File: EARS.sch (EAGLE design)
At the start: 7 parts, among them IC1 STM32L152RDT

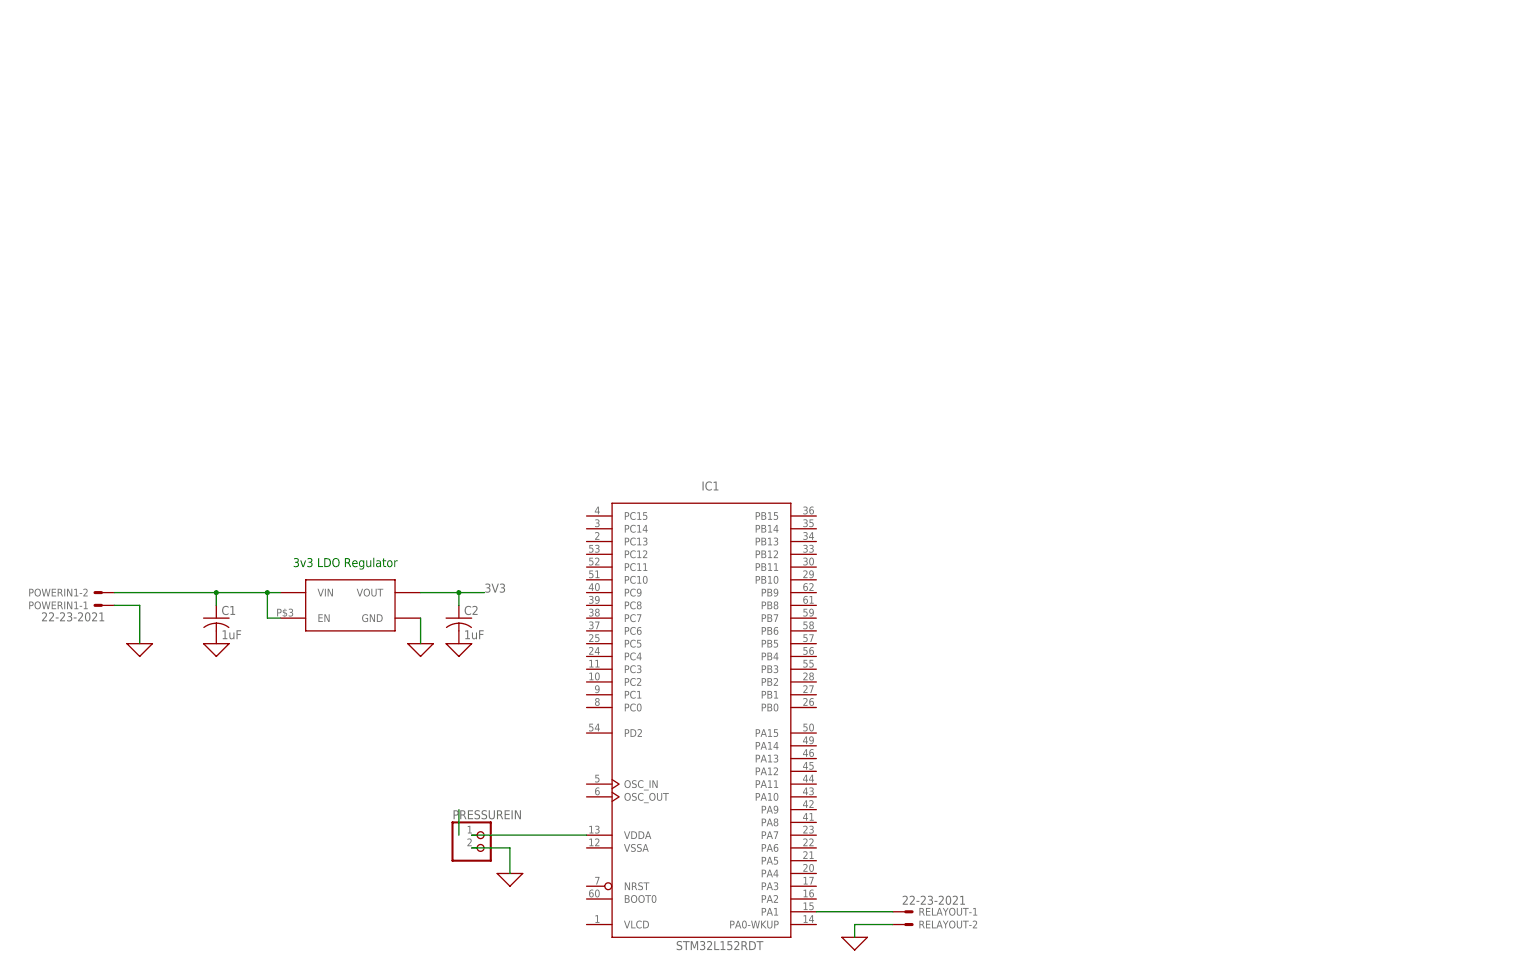
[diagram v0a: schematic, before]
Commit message: Initial Layout, fixed schematic.
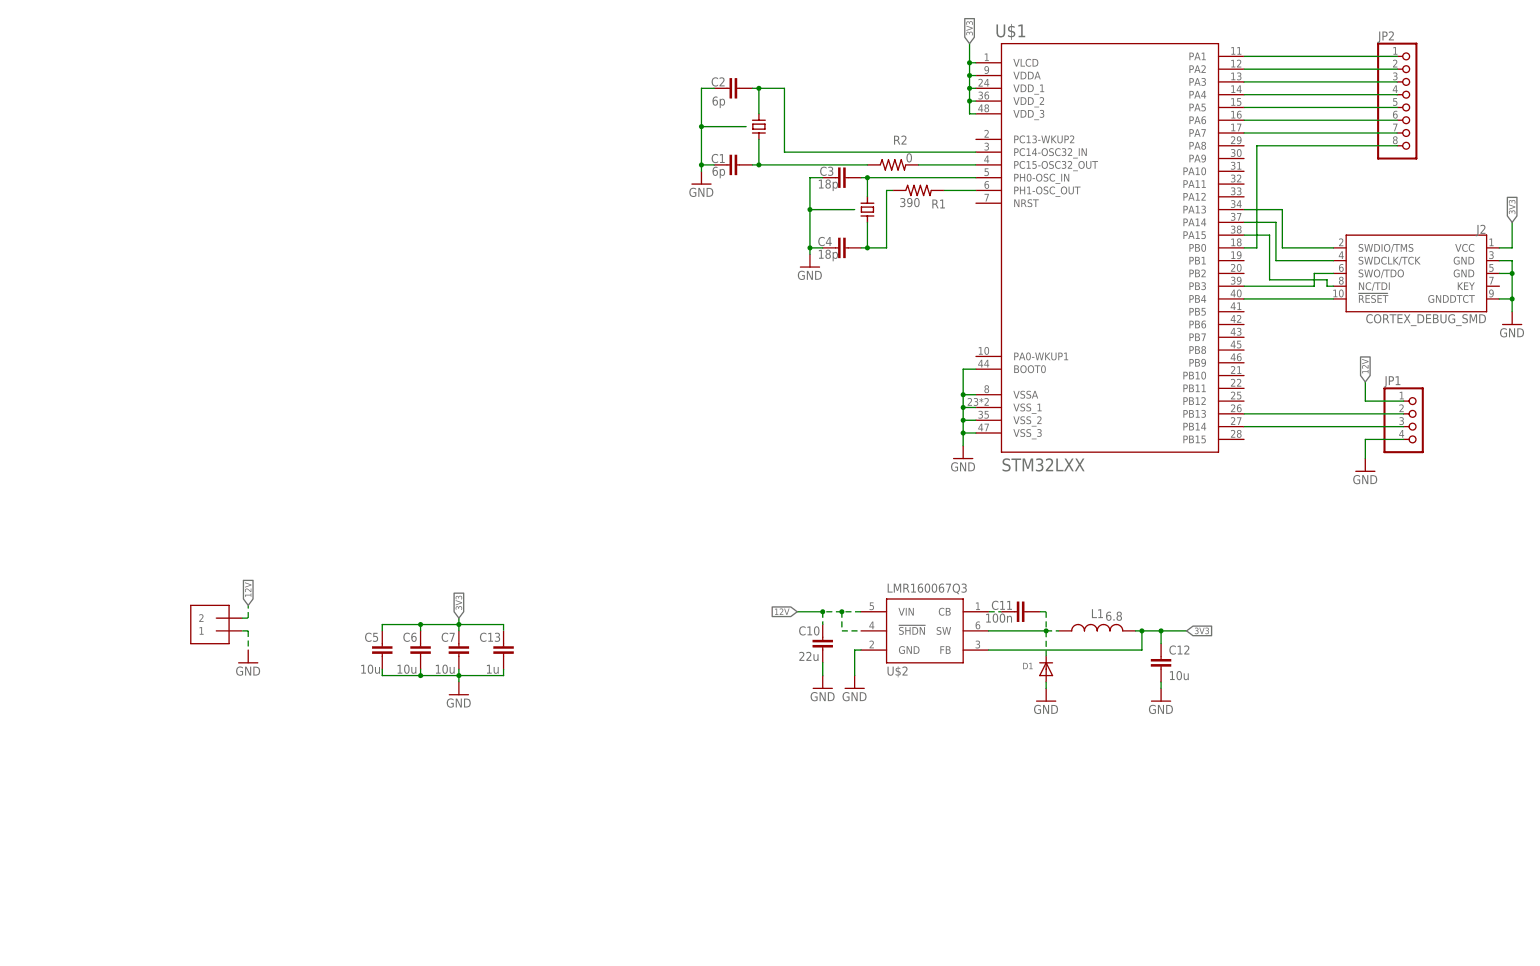
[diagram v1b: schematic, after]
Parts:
- removed 3V3REG: NCP551, EARS:NCP551
- removed IC1: STM32L152RDT, micro-stm_v3:STM32L152RDT
- removed POWERIN1, RELAYOUT: 22-23-2021, con-molex:22-23-2021
- removed PRESSUREIN: (no value), pinhead:PINHD-1X2
- added C10: 22u, rcl:C-EUC0603
- added C11: 100n, rcl:C-EUC0603
- added C12, C5, C6, C7: 10u, rcl:C-EUC0603
- added C13: 1u, rcl:C-EUC0603
- added C3, C4: 18p, rcl:C-EUC0603
- added D1: (no value), adafruit:DIODESMA
- added J1: 1X2-3.5MM, adafruit:1X2-3.5MM
- added J2: CORTEX_DEBUG_SMD, SparkFun-Connectors:CORTEX_DEBUG_SMD
- added JP1: (no value), pinhead:PINHD-1X4
- added JP2: (no value), pinhead:PINHD-1X8
- added L1: 6.8, rcl:L-USL3216C
- added R1: 390, rcl:R-US_R0603
- added R2: 0, rcl:R-US_R0603
- added U$1: STM32LXX, EARS:STM32LXX
- added U$2: LMR160067Q3, EARS:LMR160067Q3
- added X1: ECX_34G, EARS:ECX_34G
- added X2: (no value), EARS:FL0800011Q
- C1, C2: value 1uF -> 6p; device rcl:C-USC0603 -> rcl:C-EUC0603
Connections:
- removed net 0: 3V3REG.GND, C1.2, C2.2, POWERIN1-1.S, PRESSUREIN.2, RELAYOUT-2.S
- removed net N$3: IC1MCU.PA1, RELAYOUT-1.S
- removed net N$4: 3V3REG.EN, 3V3REG.VIN, C1.1, POWERIN1-2.S
- removed net N$5: IC1MCU.VDDA, PRESSUREIN.1
- new net !RESET!: J2.!RESET, U$1.PB4
- new net 12V: C10.2, J1.2, JP1.1, U$2.!SHDN!, U$2.VIN
- new net 8M0X_OUT: C4.2, R1.1, X2.C2
- new net 8MOX_IN: C3.2, U$1.PH0-OSC_IN, X2.C1
- new net GND: C1.1, C10.1, C12.2, C13.1, C2.1, C3.1, C4.1, C5.1, C6.1, C7.1, D1.A, J1.1, J2.GND@3, J2.GND@5, J2.GNDDTCT, JP1.4, U$1.BOOT0, U$1.VSSA, U$1.VSS_1, U$1.VSS_2, U$1.VSS_3, U$2.GND, X1.P$1, X2.P$1
- new net LMR_CB: C11.1, U$2.CB
- new net LMR_SW: C11.2, D1.C, L1.1, U$2.SW
- new net MCU_P4: R2.2, U$1.PC15-OSC32_OUT
- new net MCU_P6: R1.2, U$1.PH1-OSC_OUT
- new net NC: J2.NC/TDI, U$1.PA15
- new net OSC32_IN: C1.2, R2.1, X1.C2
- new net OSC32_OUT: C2.2, U$1.PC14-OSC32_IN, X1.C1
- new net P_IN1: JP2.5, U$1.PA5
- new net P_IN2: JP2.6, U$1.PA6
- new net P_IN3: JP2.7, U$1.PA7
- new net P_IN4: JP2.8, U$1.PB0
- new net P_OUT1: JP2.1, U$1.PA1
- new net P_OUT2: JP2.2, U$1.PA2
- new net P_OUT3: JP2.3, U$1.PA3
- new net P_OUT4: JP2.4, U$1.PA4
- new net SOL_1: JP1.2, U$1.PB13
- new net SOL_2: JP1.3, U$1.PB14
- new net SWDCLK: J2.SWDCLK/TCK, U$1.PA14
- new net SWDIO: J2.SWDIO/TMS, U$1.PA13
- new net SWO: J2.SWO/TDO, U$1.PB3
- net 3V3: now also C12.1, C13.2, C5.2, C6.2, C7.2, J2.VCC, L1.2, U$1.VDDA, U$1.VDD_1, U$1.VDD_2, U$1.VDD_3, U$1.VLCD, U$2.FB; no longer 3V3REG.VOUT, C2.1
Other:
- note added: "12v-3.3v DC-DC Regulator Diode Breakdown 15V"
- note added: "MCU Power Suppy 1uF caps across VDDA-VDDS 10uF Caps across VDD* (1-3)"
- note removed: "3v3 LDO Regulator"
- moved on the sheet: C1, C2
